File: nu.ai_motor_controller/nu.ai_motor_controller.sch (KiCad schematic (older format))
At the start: 18 parts

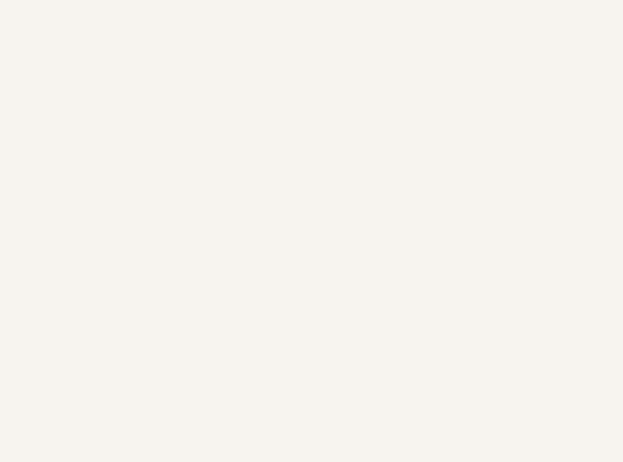
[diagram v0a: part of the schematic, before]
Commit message: automated commit
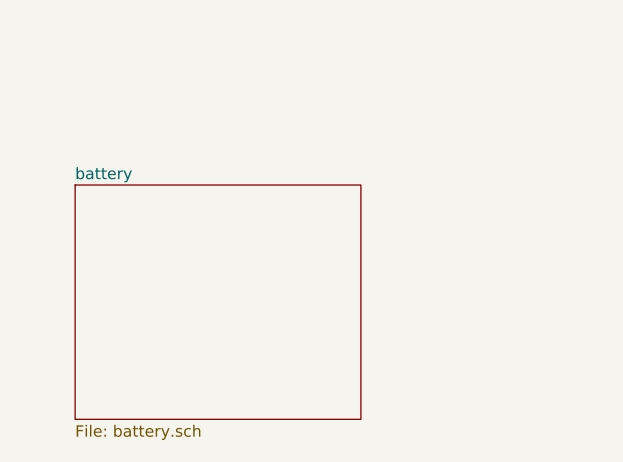
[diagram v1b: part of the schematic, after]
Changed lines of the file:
@@
 $Descr A4 11693 8268
 encoding utf-8
-Sheet 1 4
+Sheet 1 5
 Title ""
 Date ""
@@
 Wire Wire Line
 	6000 2800 5575 2800
+$Sheet
+S 1525 3325 1250 1025
+U 5C5AE643
+F0 "battery" 50
+F1 "battery.sch" 50
+$EndSheet
 $EndSCHEMATC
